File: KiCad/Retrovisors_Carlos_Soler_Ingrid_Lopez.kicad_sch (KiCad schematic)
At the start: 20 parts, among them J1 Conn_01x02, J2 Conn_01x03, J3 Conn_01x05, SW1 SW_DPST_x2, U1 PIC32MX250F128B-50I/SO, Y1 Crystal

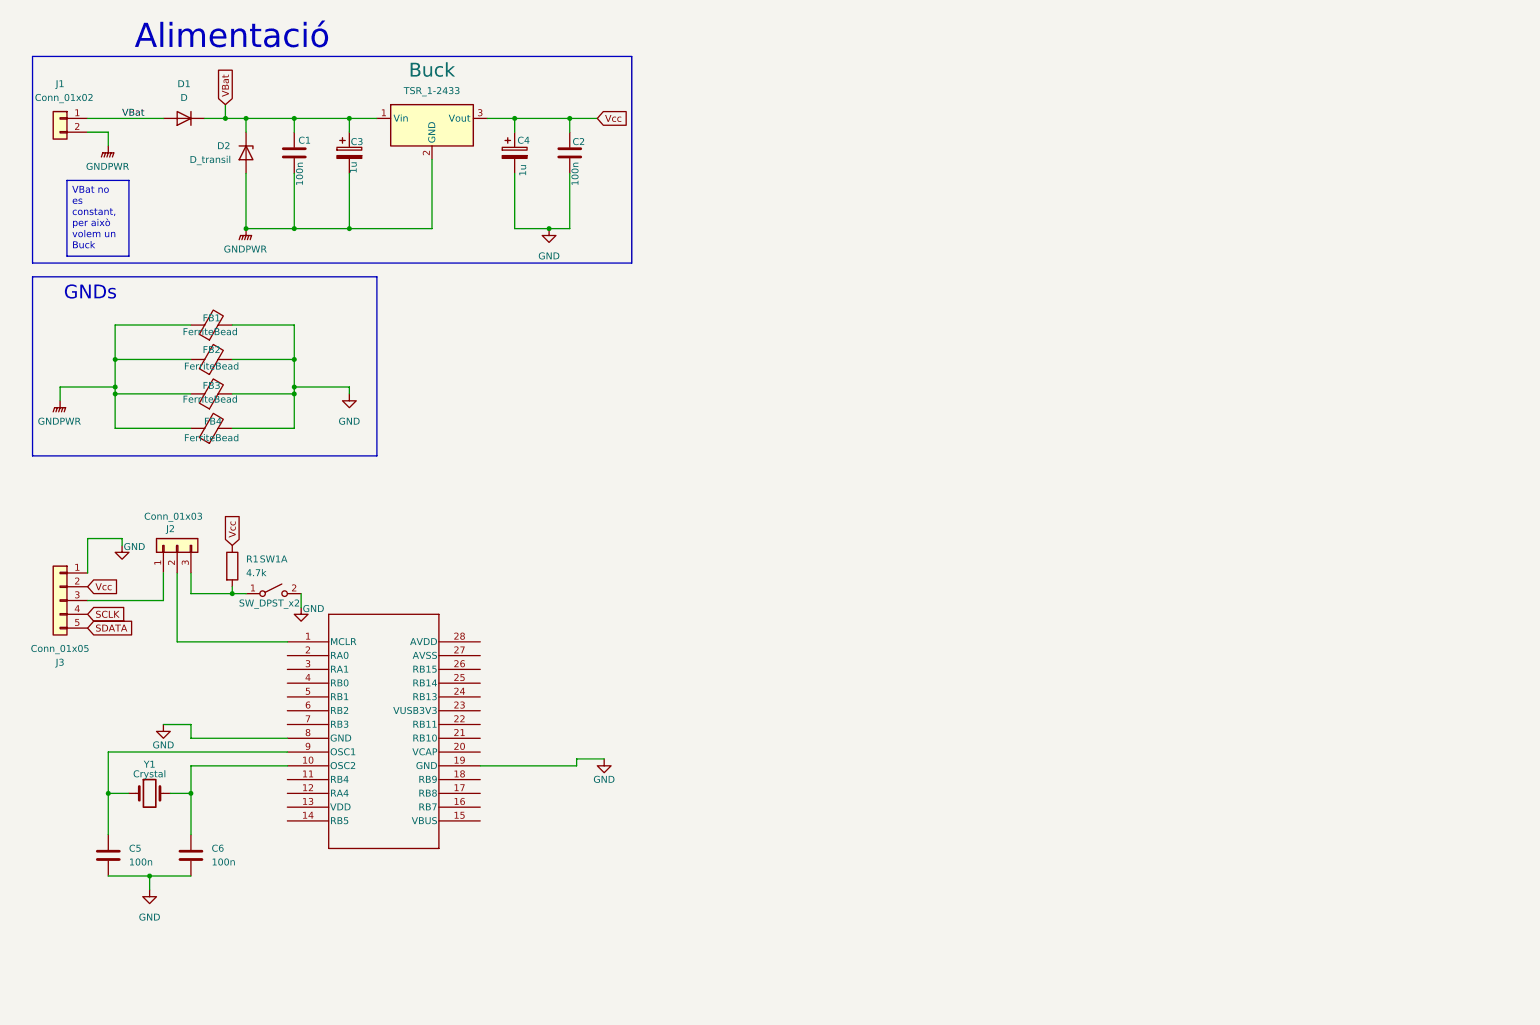
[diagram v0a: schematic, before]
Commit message: microcontrolador i driver
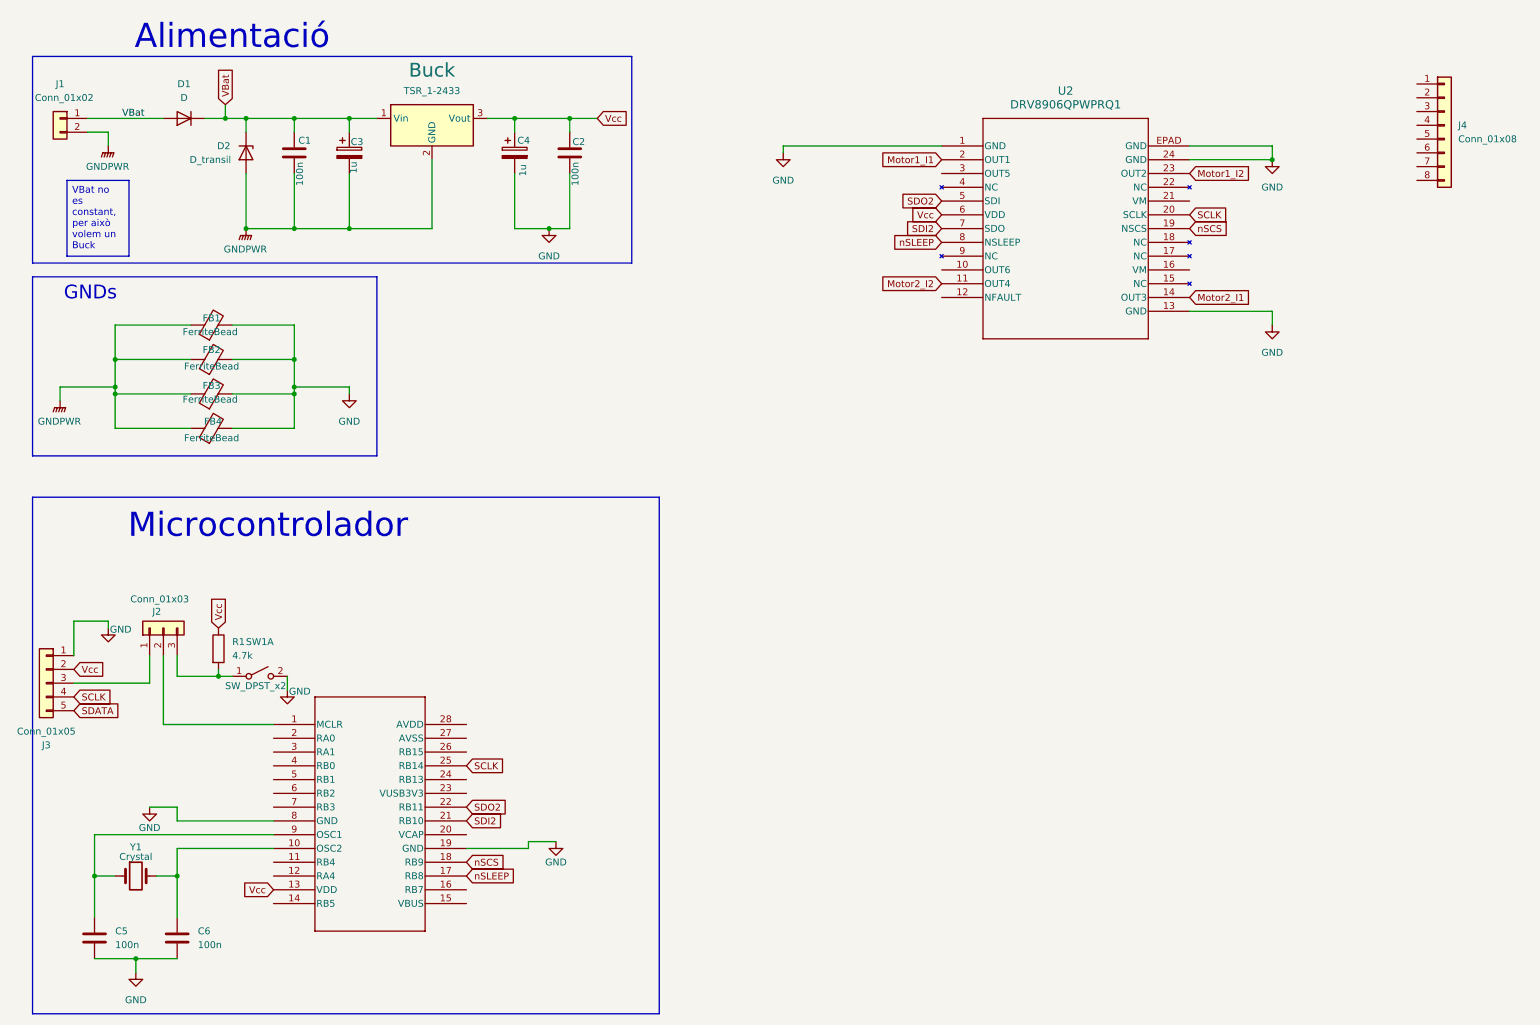
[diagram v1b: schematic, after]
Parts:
- added J4: Conn_01x08, symbol Connector_Generic:Conn_01x08
- added U2: DRV8906QPWPRQ1, HTSSOP24_PWP_TEX, symbol Drivers_motors_xy:DRV8906QPWPRQ1
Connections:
- net GND: now also U2.1 (GND), U2.13 (GND), U2.24 (GND), U2.EPAD (GND)
- net SCLK: now also U1.25 (RB14), U2.20 (SCLK)
- net Vcc: now also U1.13 (VDD), U2.6 (VDD)
- net nSLEEP: now reaches U1.17 (RB8)
- net nSLEEP: now also U2.8 (NSLEEP)
- net nSCS: now reaches U1.18 (RB9)
- net nSCS: now also U2.19 (NSCS)
- net SDI2: now reaches U1.21 (RB10)
- net SDI2: now also U2.7 (SDO)
- net SDO2: now reaches U1.22 (RB11)
- net SDO2: now also U2.5 (SDI)
- new net Motor1_I1: U2.2 (OUT1)
- new net Motor1_I2: U2.23 (OUT2)
- new net Motor2_I1: U2.14 (OUT3)
- new net Motor2_I2: U2.11 (OUT4)
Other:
- note added: "Microcontrolador"
- moved on the sheet: C5, C6, J2, J3, R1, SW1A, Y1
